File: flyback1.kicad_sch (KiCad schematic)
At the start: 38 parts, among them IC1 INN3649C-H606-TL, J2 Conn_01x02_Socket, Q1 100V, T1 P0544NL

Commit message: finalized schematic
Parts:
- added C2.3, C2.4: 0.25u, symbol Device:C
- added R11.2, R11.3, R11.4: 40ohm, symbol Device:R
- added R5.3, R5.4: 40, symbol Device:R
- added R8.2, R8.3: 8.1k, symbol Device:R
- C2.1: value 82u -> 40u; Voltage 450V -> 900
- C2.2: value 82u -> 0.25u; Voltage 450V -> 900
- R11.1: renamed from R11; value 10 -> 40ohm
- R5.1: renamed from R5; value 20 -> 40
- R5.2: renamed from R6; value 20 -> 40
- R8.1: renamed from R8; value 2.7k -> 8.1k
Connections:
- net BPP: now also R8.2.2, R8.3.2
- net Earth: now also C2.1.2, C2.3.2, C2.4.2
- net T6: now also R11.2.1, R11.3.1, R11.4.1
- net VCC: now also C2.2.1, C2.3.1, C2.4.1
- net at C4.1, R5.1.1, R5.2.1: now also R5.3.1, R5.4.1
- net at D1.1 (K), R5.1.2, R5.2.2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: now also R5.3.2, R5.4.2
- net at C7.1, D4.2 (A), R11.1.2: now also R11.2.2, R11.3.2, R11.4.2
- net at C5.1, D2.1 (K), R8.1.1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: now also R8.2.1, R8.3.1
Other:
- moved on the sheet: C10, C11, C12, C13, C15, C16, C2.1, C4, C5, C6, C7, C8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

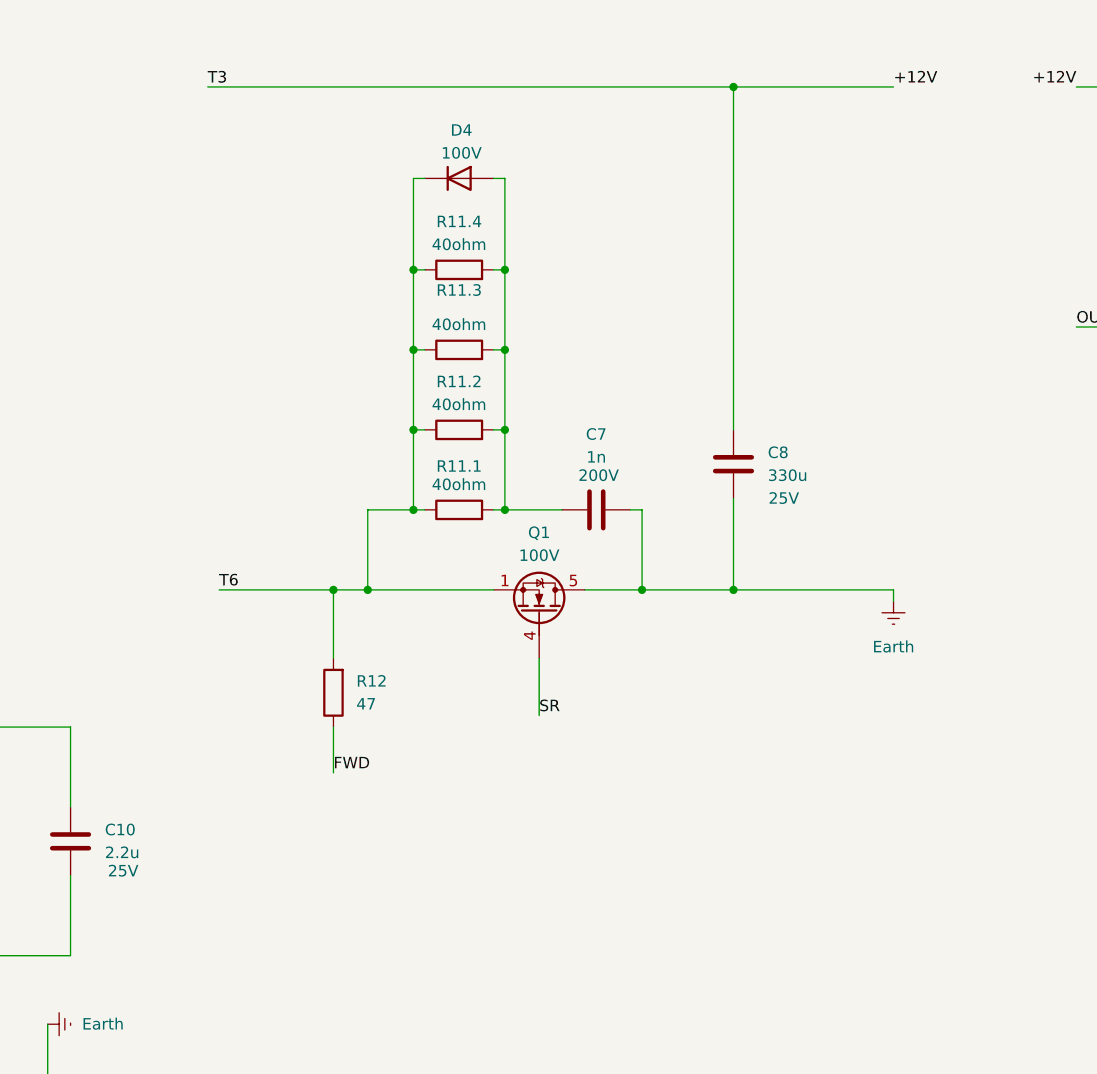
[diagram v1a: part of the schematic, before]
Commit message: R2, D5, R1 added
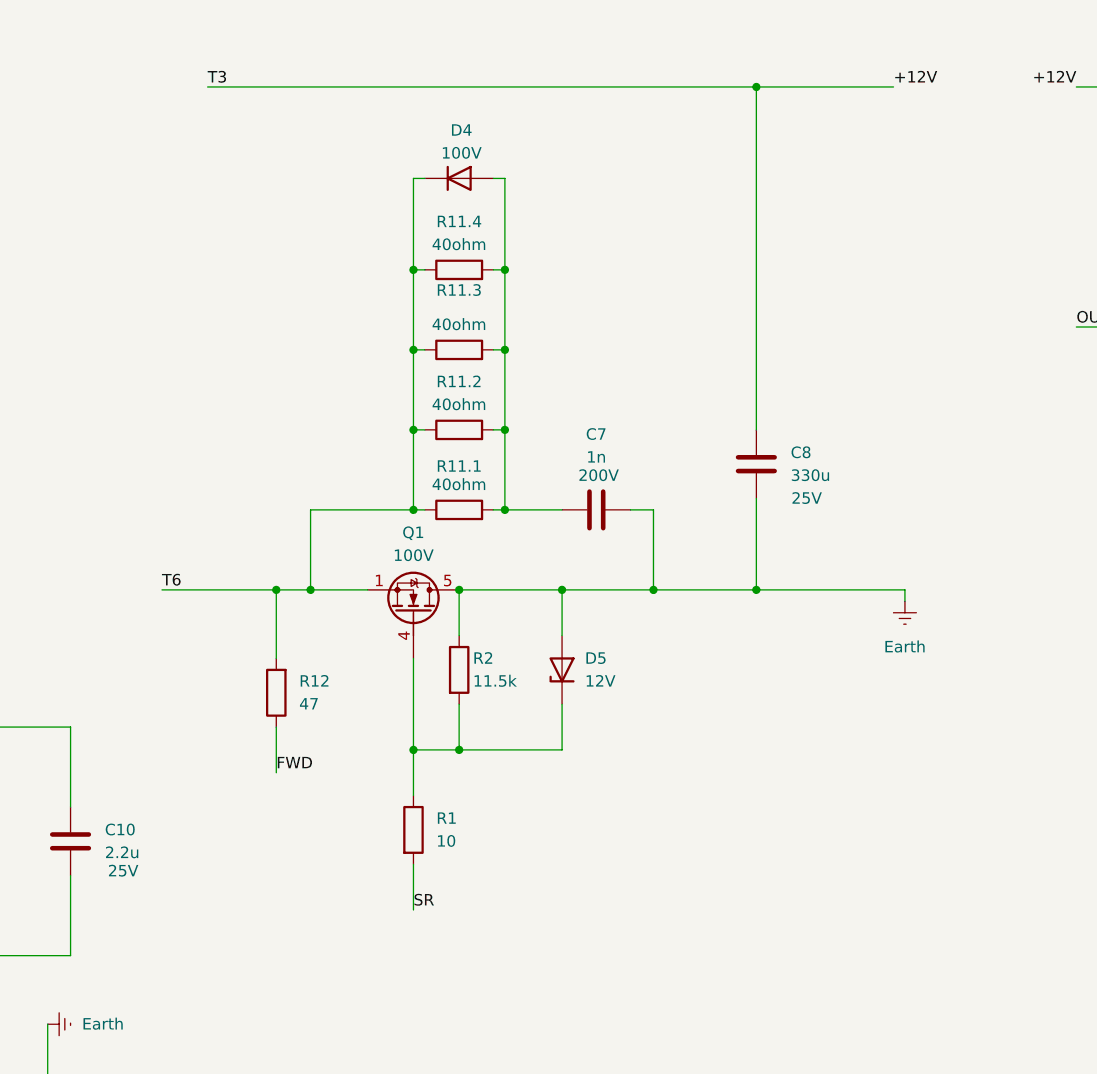
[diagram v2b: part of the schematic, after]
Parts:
- added D5: 12V, symbol Device:D_Zener
- added R1: 10, symbol Device:R
- added R2: 11.5k, symbol Device:R
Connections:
- net Earth: now also D5.2 (A), R2.1
- net SR: now also R1.2; no longer Q1.4 (G)
- new net: D5.1 (K), Q1.4 (G), R1.1, R2.2
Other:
- moved on the sheet: C8, Q1, R12
